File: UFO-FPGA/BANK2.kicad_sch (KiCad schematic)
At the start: 11 parts, among them U1 ICE40HX8K-BG121

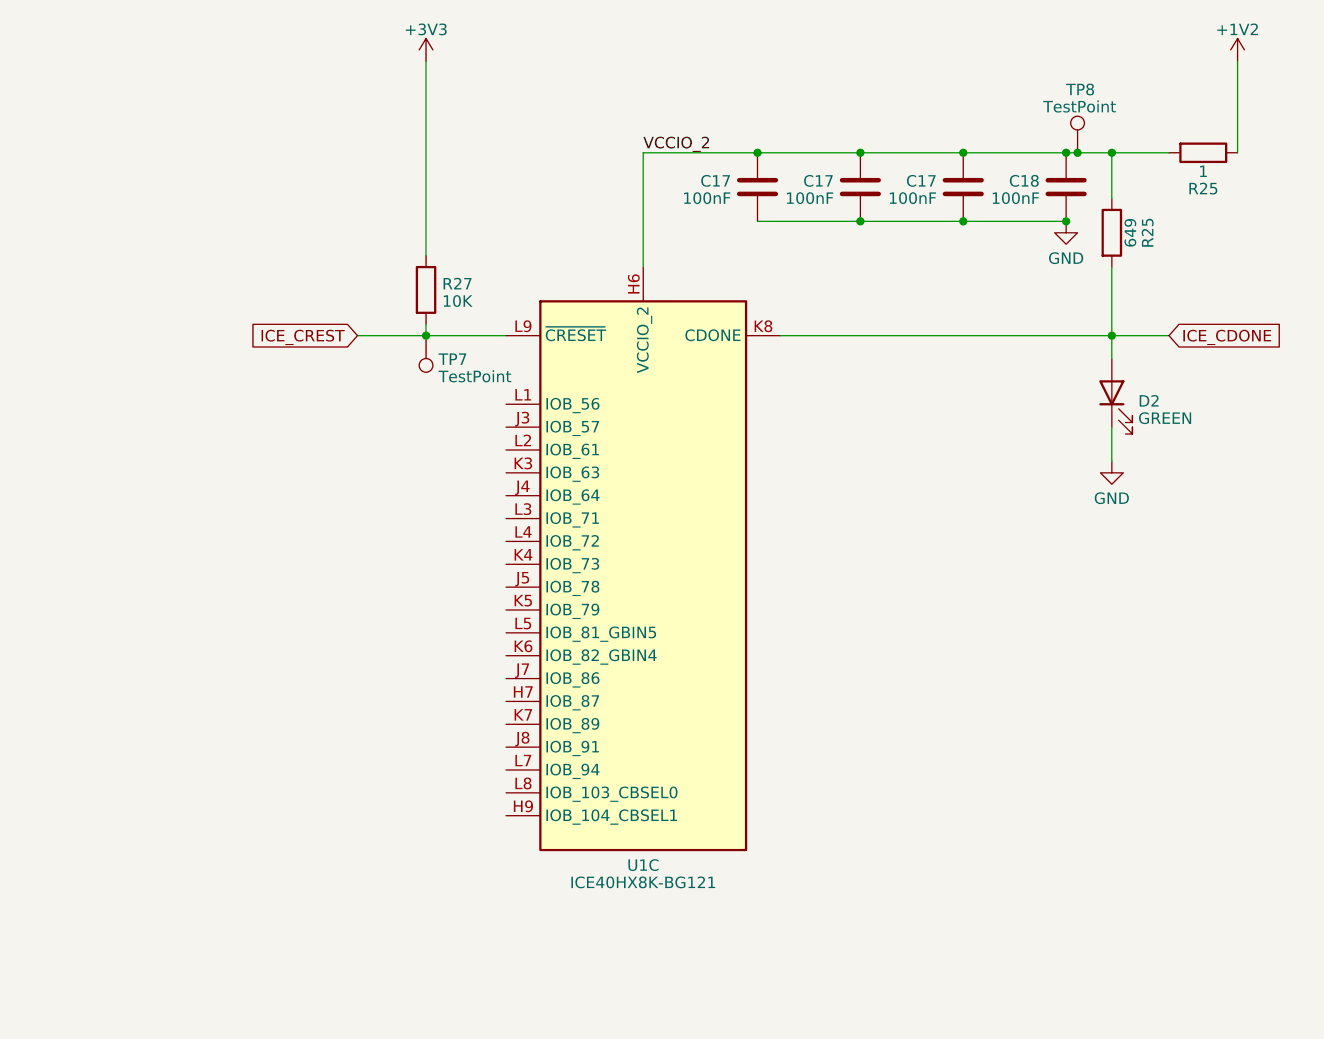
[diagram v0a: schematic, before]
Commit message: IO and power
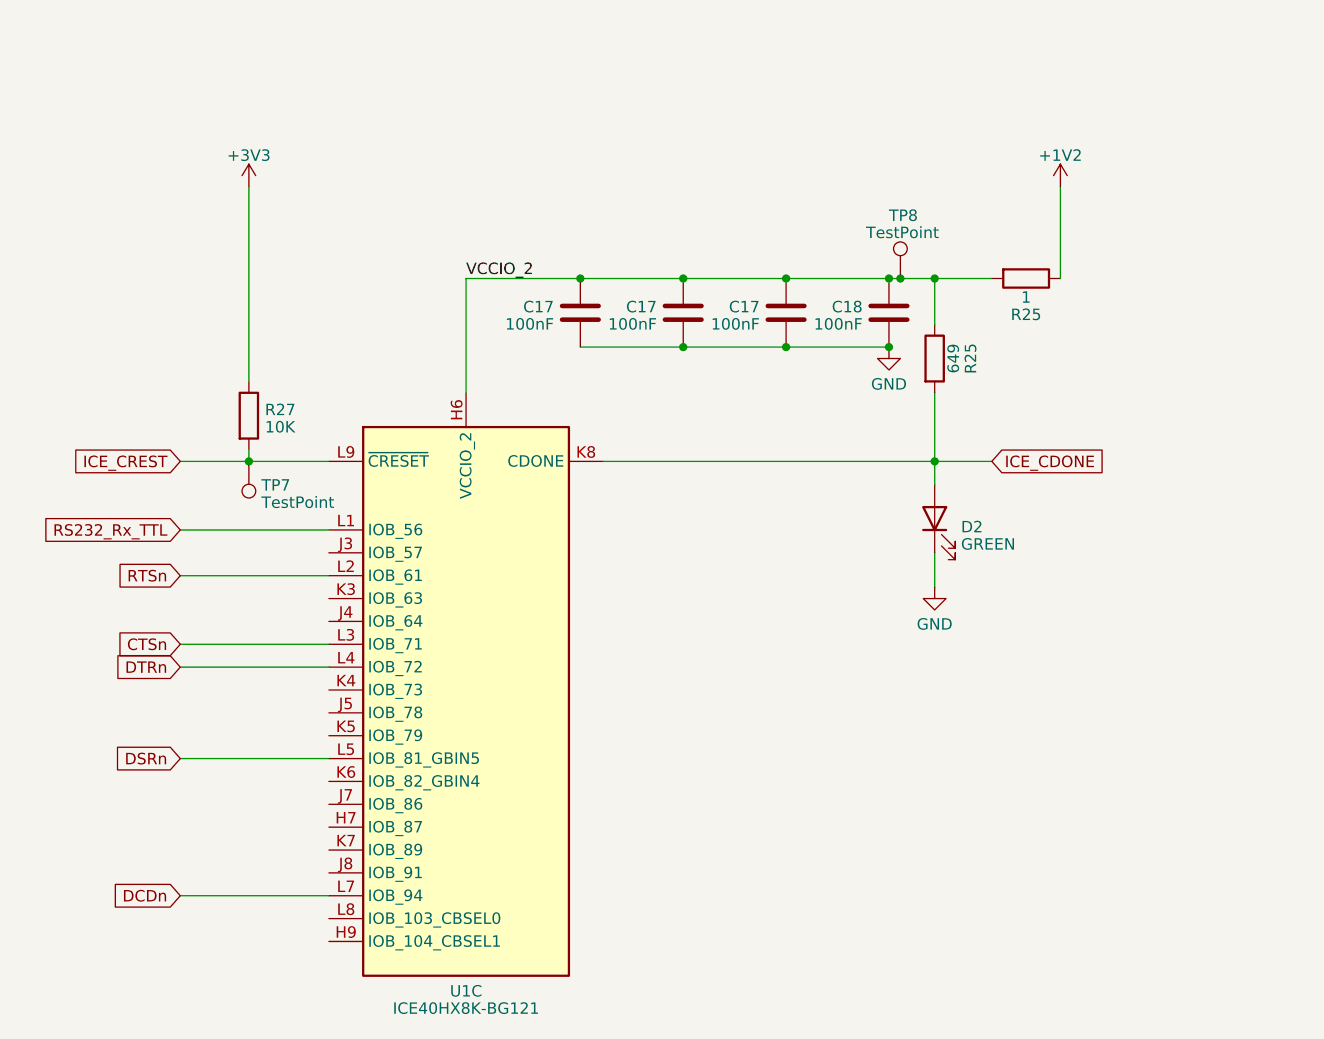
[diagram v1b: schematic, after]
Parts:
- removed C17 (x3): 100nF, symbol Device:C
- removed R25: 649, symbol Device:R
- removed R25: 1, symbol Device:R
- added C17 (x3): 100nF, symbol Device:C
- added R25: 649, symbol Device:R
- added R25: 1, symbol Device:R
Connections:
- net +1V2: now also R25.1
- net GND: now also C17.2, C17.2, C17.2
- net ICE_CDONE: now also R25.2
- net VCCIO_2: now also C17.1, C17.1, C17.1, R25.1, R25.2
- net RS232_Rx_TTL: now reaches U1.L1 (IOB_56)
- net RTSn: now reaches U1.L2 (IOB_61)
- net CTSn: now reaches U1.L3 (IOB_71)
- net DTRn: now reaches U1.L4 (IOB_72)
- net DSRn: now reaches U1.L5 (IOB_81_GBIN5)
- net DCDn: now reaches U1.L7 (IOB_94)
